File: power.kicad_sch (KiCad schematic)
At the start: 6 parts, among them IC2 BQ21080YBGR, U2 TPS631000DRLR, U3 TPS62840DLCR

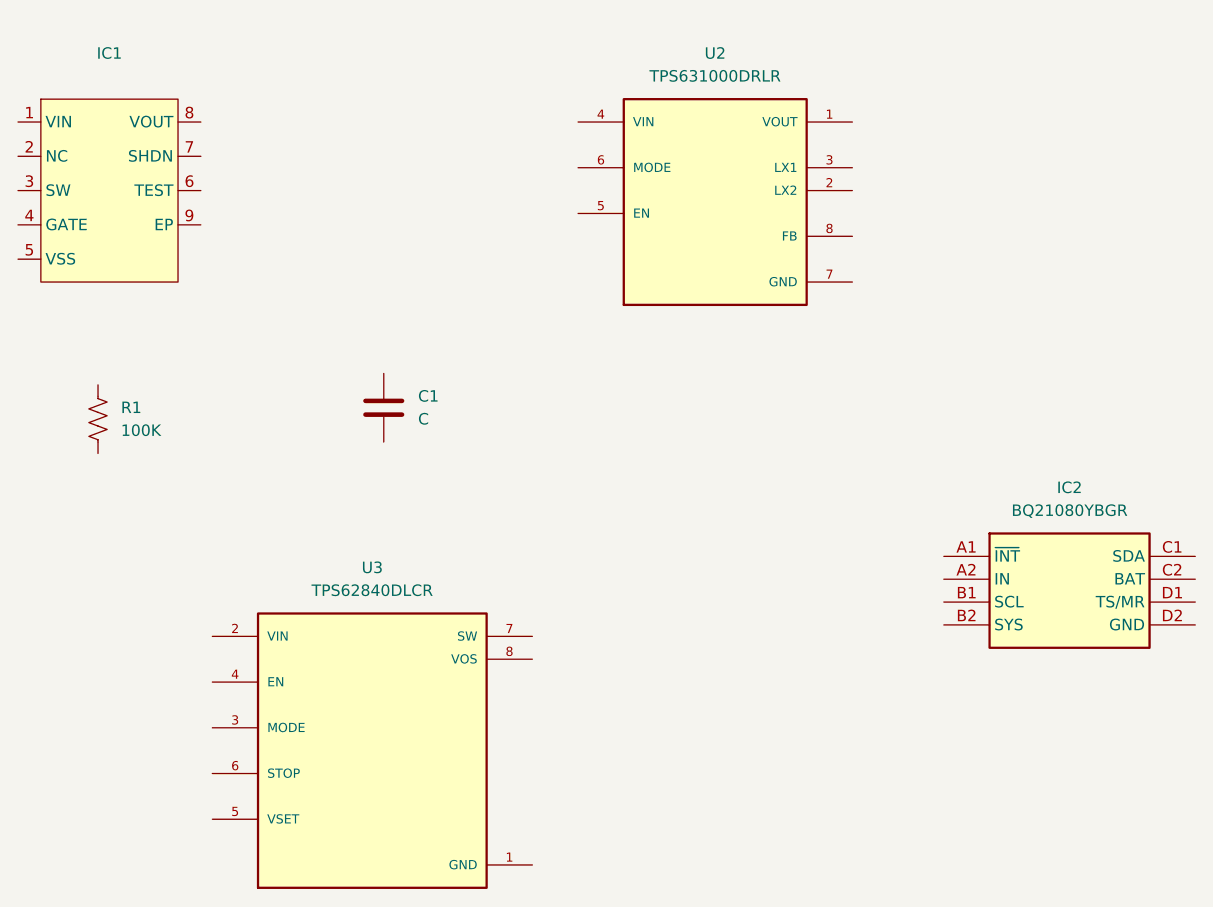
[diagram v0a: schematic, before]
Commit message: Update
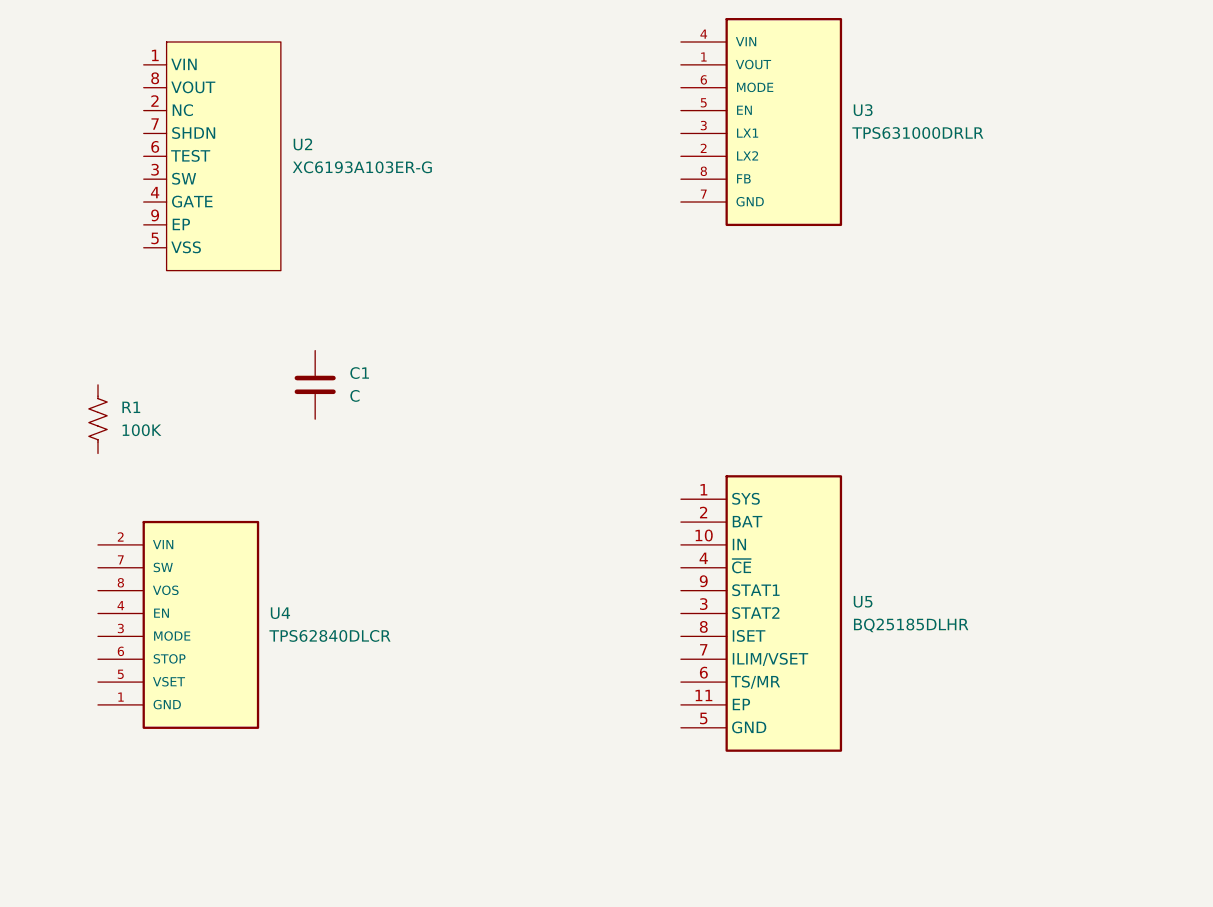
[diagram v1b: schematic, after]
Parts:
- removed IC1: ~, footprints:SON40P150X150X50-9N, symbol XC6193:XC6193A103ER-G
- removed IC2: BQ21080YBGR, footprints:BGA8C40P2X4_100X155X50, symbol BQ21080YBGR:BQ21080YBGR
- removed U2: TPS631000DRLR, footprints:SOT50P160X60-8N, symbol TPS631000DRLR:TPS631000DRLR
- removed U3: TPS62840DLCR, footprints:SON50P200X150X100-8N, symbol TPS62840DLCR:TPS62840DLCR
- added U2: XC6193A103ER-G, footprints:SON40P150X150X50-9N, symbol XC6193:XC6193A103ER-G
- added U3: TPS631000DRLR, footprints:SOT50P160X60-8N, symbol TPS631000DRLR:TPS631000DRLR
- added U4: TPS62840DLCR, footprints:SON50P200X150X100-8N, symbol TPS62840DLCR:TPS62840DLCR
- added U5: BQ25185DLHR, footprints:SON40P220X200X80-11N, symbol BQ25185DLHR:BQ25185DLHR
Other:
- moved on the sheet: C1

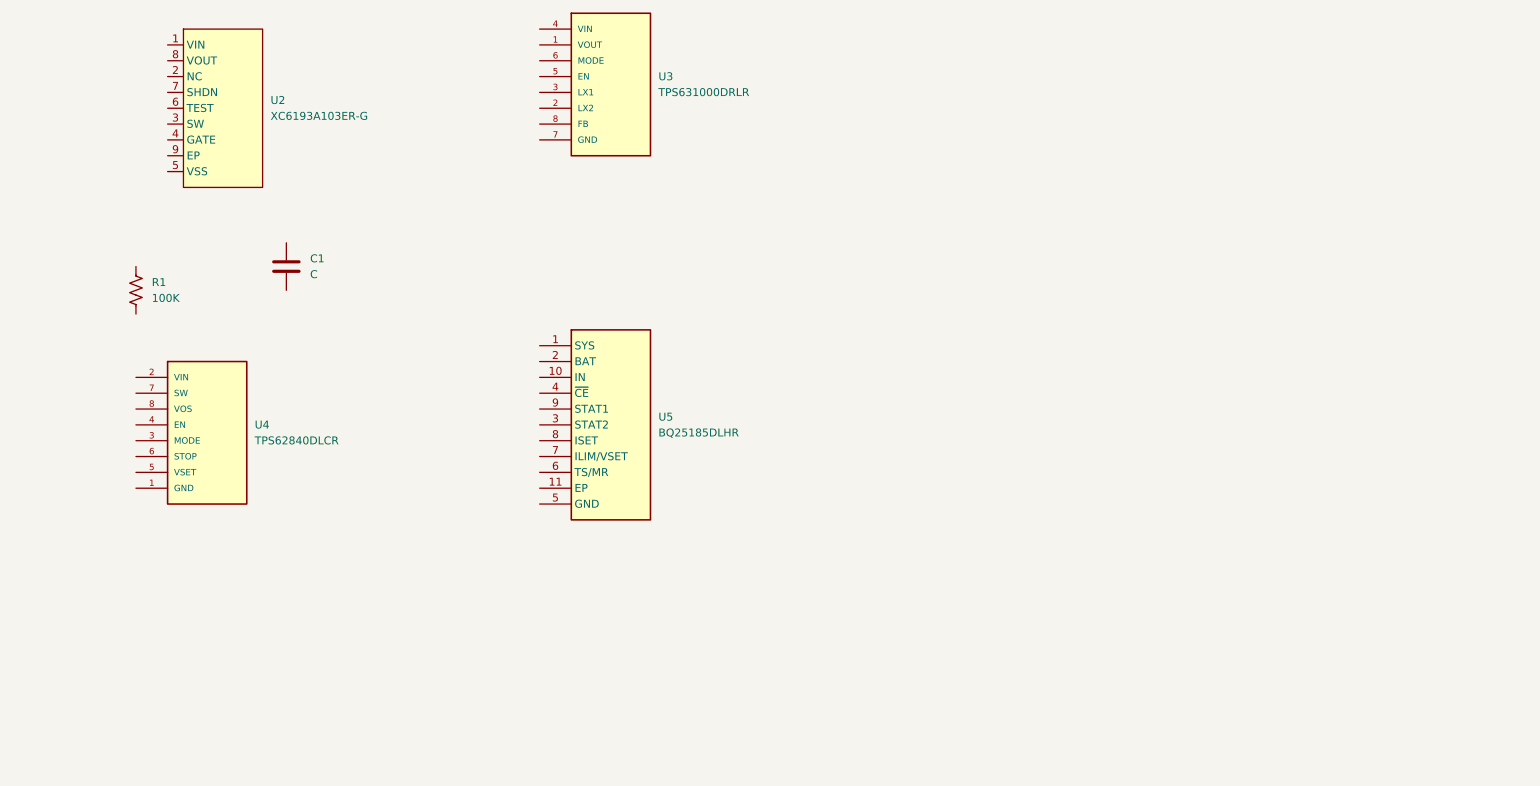
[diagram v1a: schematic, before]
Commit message: Update
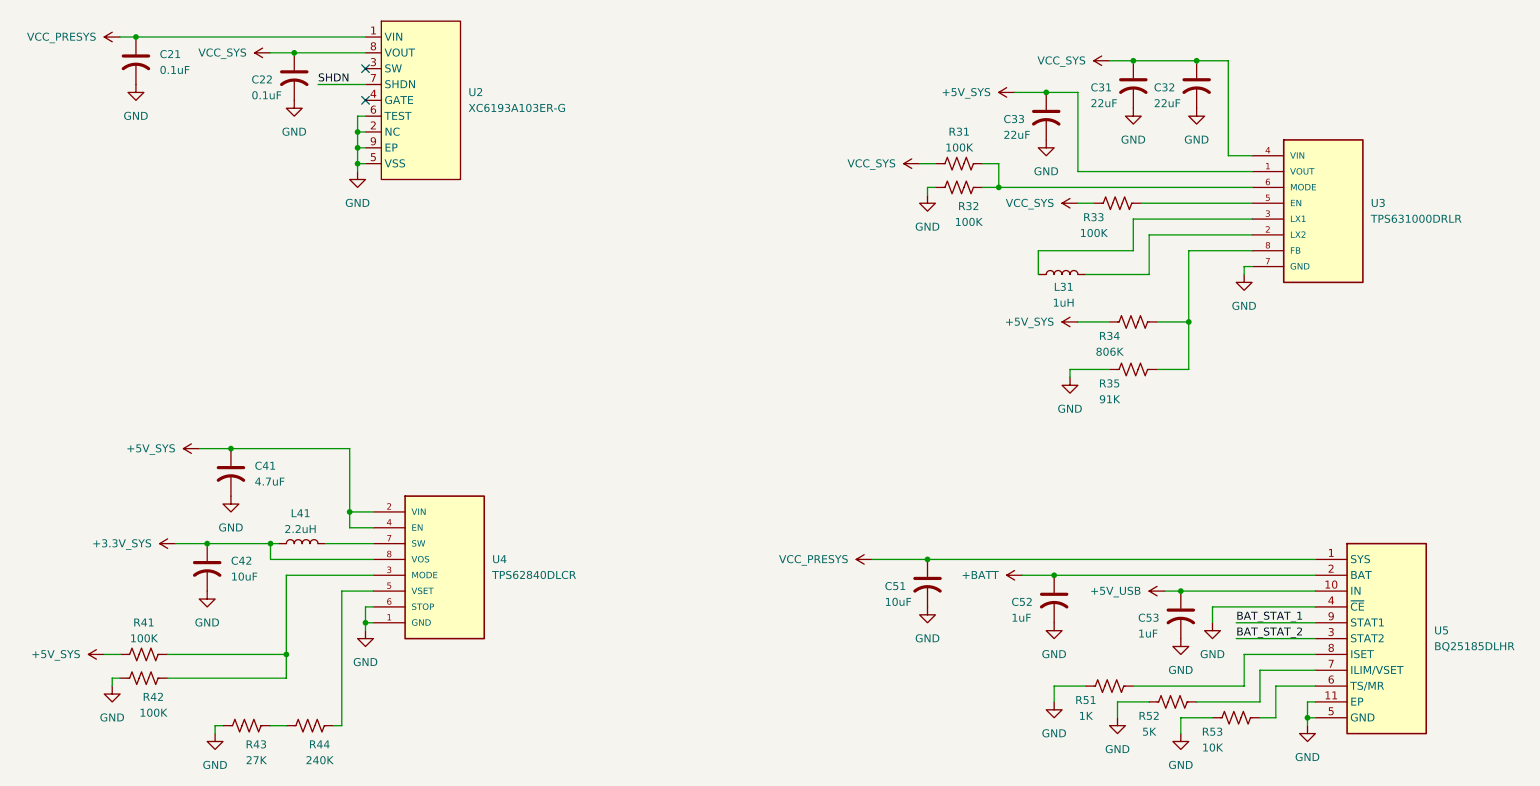
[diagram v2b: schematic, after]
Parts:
- removed C1: C, Capacitor_SMD:C_0402_1005Metric, symbol Device:C
- removed R1: 100K, Resistor_SMD:R_0402_1005Metric, symbol Device:R_US
- added C21, C22: 0.1uF, Capacitor_SMD:C_0402_1005Metric, symbol Device:C_US
- added C31, C32, C33: 22uF, Capacitor_SMD:C_0402_1005Metric, symbol Device:C_US
- added C41: 4.7uF, Capacitor_SMD:C_0402_1005Metric, symbol Device:C_US
- added C42, C51: 10uF, Capacitor_SMD:C_0402_1005Metric, symbol Device:C_US
- added C52, C53: 1uF, Capacitor_SMD:C_0402_1005Metric, symbol Device:C_US
- added L31: 1uH, Inductor_SMD:L_0402_1005Metric, symbol Device:L
- added L41: 2.2uH, Inductor_SMD:L_0402_1005Metric, symbol Device:L
- added R31, R32, R33, R41, R42: 100K, Resistor_SMD:R_0402_1005Metric, symbol Device:R_US
- added R34: 806K, Resistor_SMD:R_0402_1005Metric, symbol Device:R_US
- added R35: 91K, Resistor_SMD:R_0402_1005Metric, symbol Device:R_US
- added R43: 27K, Resistor_SMD:R_0402_1005Metric, symbol Device:R_US
- added R44: 240K, Resistor_SMD:R_0402_1005Metric, symbol Device:R_US
- added R51: 1K, Resistor_SMD:R_0402_1005Metric, symbol Device:R_US
- added R52: 5K, Resistor_SMD:R_0402_1005Metric, symbol Device:R_US
- added R53: 10K, Resistor_SMD:R_0402_1005Metric, symbol Device:R_US
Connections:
- net GND: now reaches U4.1 (GND)
- net GND: now also U2.2 (NC), U2.5 (VSS), U2.6 (TEST), U2.9 (EP), U3.7 (GND), U4.6 (STOP), U5.11 (EP), U5.4 (~{CE}), U5.5 (GND), C21.2, C22.2, C31.2, C32.2, C33.2, C41.2, C42.2, C51.2, C52.2, C53.2, R32.2, R35.2, R42.2, R43.2, R51.2, R52.2, R53.2
- net +5V_SYS: now reaches U4.2 (VIN)
- net +5V_SYS: now also U3.1 (VOUT), U4.4 (EN), C33.1, C41.1, R34.2, R41.2
- net at U4.3 (MODE): now also R41.1, R42.1
- net at U4.5 (VSET): now also R44.1
- net at U4.7 (SW): now also L41.2
- net +3.3V_SYS: now reaches U4.8 (VOS)
- net +3.3V_SYS: now also C42.1, L41.1
- net VCC_PRESYS: now reaches U5.1 (SYS)
- net VCC_PRESYS: now also U2.1 (VIN), C21.1, C51.1
- net +5V_USB: now reaches U5.10 (IN)
- net +5V_USB: now also C53.1
- net +BATT: now reaches U5.2 (BAT)
- net +BATT: now also C52.1
- net BAT_STAT_2: now reaches U5.3 (STAT2)
- net at U5.6 (TS/MR): now also R53.1
- net at U5.7 (ILIM/VSET): now also R52.1
- net at U5.8 (ISET): now also R51.1
- net BAT_STAT_1: now reaches U5.9 (STAT1)
- net SHDN: now reaches U2.7 (SHDN)
- net VCC_SYS: now reaches U2.8 (VOUT)
- net VCC_SYS: now also U3.4 (VIN), C22.1, C31.1, C32.1, R31.2, R33.2
- net at U3.2 (LX2): now also L31.2
- net at U3.3 (LX1): now also L31.1
- net at U3.5 (EN): now also R33.1
- net at U3.6 (MODE): now also R31.1, R32.1
- net at U3.8 (FB): now also R34.1, R35.1
- new net: R43.1, R44.2
- no-connect marks 0 -> 2
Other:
- moved on the sheet: U2, U3, U4, U5
